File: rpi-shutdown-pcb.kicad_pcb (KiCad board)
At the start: 2 copper layers, 40.5 x 22 mm, 16 parts, among them IC1 ATTINY85-P, P1 CONN_01X03, P2 CONN_01X02, Q1 MOSFET_N_(2N7002P,215), Q2 MOSFET_N_(2N7002P,215), Q3 SI2369DS-T1-GE3, U1 LM3480-3.3

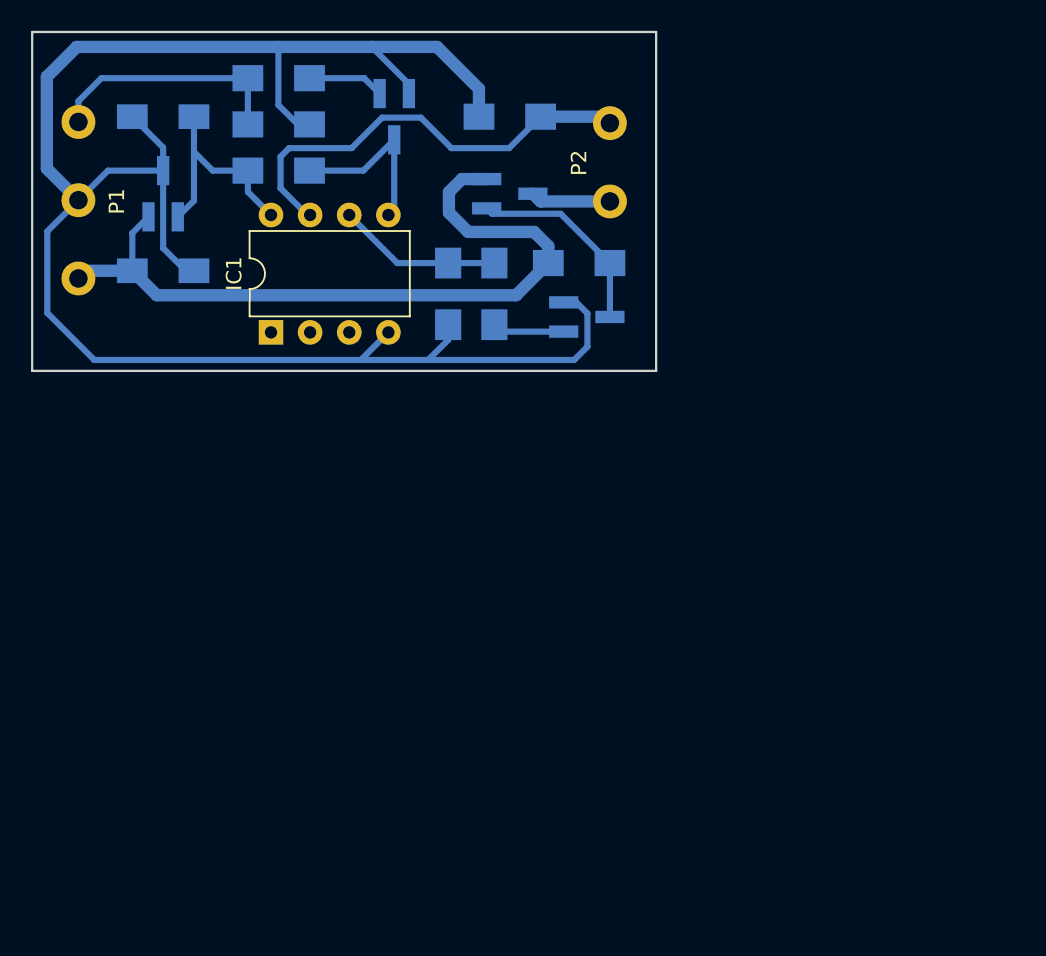
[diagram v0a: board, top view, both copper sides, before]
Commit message: Finished PCB layout.  Ready to try routing.
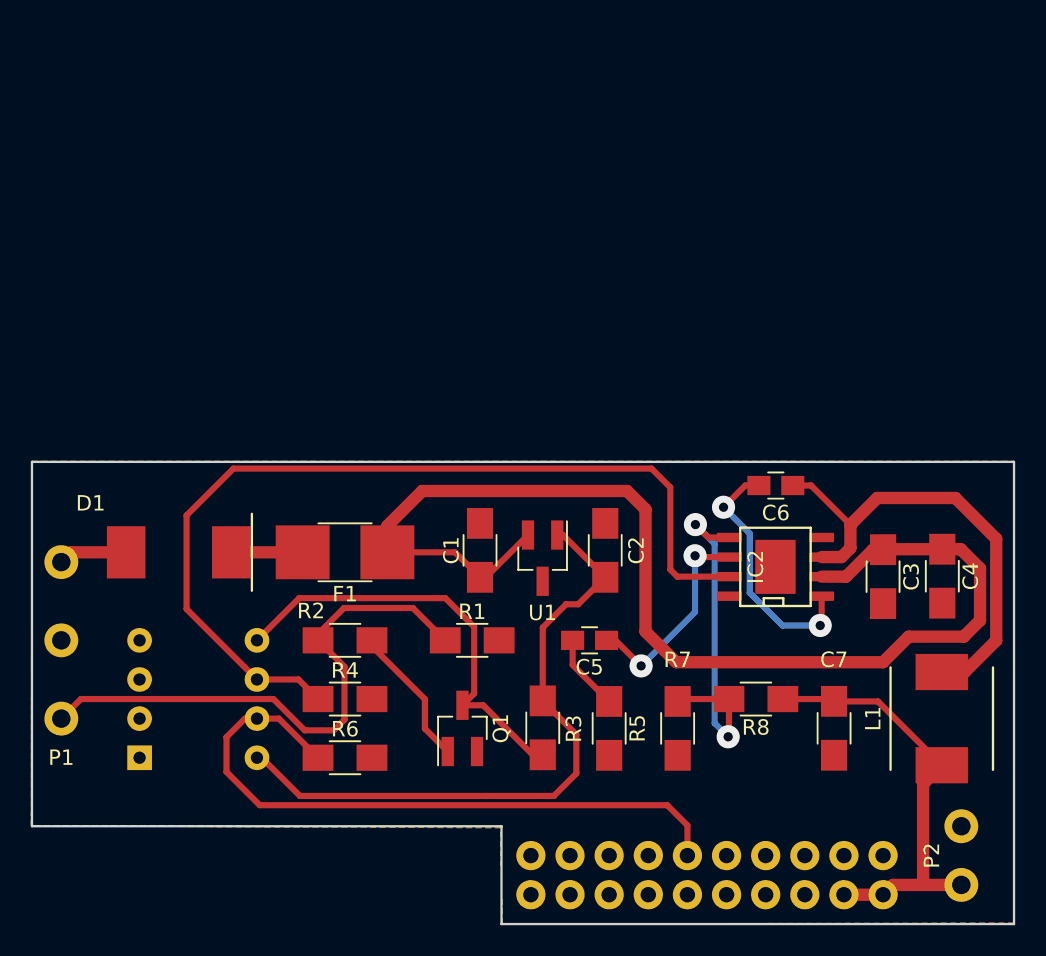
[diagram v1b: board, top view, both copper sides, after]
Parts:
- removed Q2: MOSFET_N_(2N7002P,215), TO_SOT_Packages_SMD:SOT-23_Handsoldering
- removed Q3: SI2369DS-T1-GE3, TO_SOT_Packages_SMD:SOT-23_Handsoldering
- added C3: 10uF, rpi-shutdown-pcb:R_1206_HandSoldering_(narrow), F.Cu at (189.2, 106.4)
- added C4: 10uF, rpi-shutdown-pcb:R_1206_HandSoldering_(narrow), F.Cu at (193.1, 106.3)
- added C5: 3.9nF, rpi-shutdown-pcb:C_0805_HandSoldering_(narrow), F.Cu at (170.2, 110.5)
- added C6: 10nF, rpi-shutdown-pcb:C_0805_HandSoldering_(narrow), F.Cu at (182.3, 100.4)
- added C7: 33uF, rpi-shutdown-pcb:R_1206_HandSoldering_(narrow), F.Cu at (186.1, 116.2)
- added CONN_1: CONN_02X10, rpi-shutdown-pcb:HEADER_20_PIN_FEMALE_(PPTC102LFBN-RC), B.Cu at (189.2, 124.5)
- added D1: D_Schottky, rpi-shutdown-pcb:DO-214AB, F.Cu at (143.5, 104.8)
- added F1: Polyfuse, rpi-shutdown-pcb:R_1812_HandSoldering, F.Cu at (154.3, 104.8)
- added IC2: STEP_DOWN_CONVERTER_(MP2307), rpi-shutdown-pcb:SOIC8N_(EXPOSED_PAD), F.Cu at (182.2, 105.7)
- added L1: 10uH, rpi-shutdown-pcb:INDUCTOR_10uH_(ASPI-0630LR), F.Cu at (193.0, 115.6)
- added R8: 10k, rpi-shutdown-pcb:R_1206_HandSoldering_(narrow), F.Cu at (181.0, 114.3)
- C1, C2: footprint Capacitors_SMD:C_1206_HandSoldering -> rpi-shutdown-pcb:R_1206_HandSoldering_(narrow); moved to F.Cu
- IC1: moved to B.Cu
- Q1, U1: moved to F.Cu
- R1, R2, R3, R4, R6: footprint Resistors_SMD:R_1206_HandSoldering -> rpi-shutdown-pcb:R_1206_HandSoldering_(narrow); moved to F.Cu
- R5: value 150 -> 6.8K; footprint Resistors_SMD:R_1206_HandSoldering -> rpi-shutdown-pcb:R_1206_HandSoldering_(narrow); moved to F.Cu
- R7: value 0.1 -> 2.2K; footprint Resistors_SMD:R_1206_HandSoldering -> rpi-shutdown-pcb:R_1206_HandSoldering_(narrow); moved to F.Cu
- moved P2 49.9 mm to (194.3, 126.4)
- moved R7 41.2 mm to (175.9, 116.2), turned to 270 degrees
- moved C2 40.2 mm to (171.2, 104.6), turned to 90 degrees
- moved R3 40.0 mm to (167.1, 116.2), turned to 270 degrees
- moved Q1 40.0 mm to (161.9, 116.2), turned to 90 degrees
- moved R2 36.7 mm to (154.3, 110.5)
- moved R1 35.8 mm to (162.6, 110.5)
- moved R6 35.5 mm to (154.3, 118.1)
- moved U1 34.2 mm to (167.1, 105.2), turned to 270 degrees
- moved R5 29.2 mm to (171.4, 116.2), turned to 270 degrees
- moved IC1 28.9 mm to (141.0, 118.1), turned to 0 degrees
- moved C1 27.4 mm to (163.1, 104.6), turned to 90 degrees
- moved R4 27.1 mm to (154.3, 114.3), turned to 0 degrees
- moved P1 18.4 mm to (135.9, 105.4), turned to 270 degrees
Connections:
- IC1 pad 7: Net-(IC1-Pad7) -> Net-(CONN_1-Pad11)
- P1 pad 1: Net-(C1-Pad1) -> Net-(D1-Pad2)
- P2 pad 2: Net-(IC1-Pad7) -> GND
- R5 pad 2: Net-(IC1-Pad6) -> GND
- R6 pad 1: Net-(C1-Pad1) -> Net-(CONN_1-Pad11)
- R6 pad 2: Net-(Q2-Pad3) -> GND
- R7 pad 1: GND -> Net-(IC2-Pad5)
- R7 pad 2: Net-(IC1-Pad7) -> GND
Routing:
- net GND: track 124.0 -> 1.33 mm
- net Net-(IC1-Pad6): track 10.7 -> 59.6 mm
- net Net-(CONN_1-Pad11): track 0.00 -> 43.1 mm
- net Net-(C6-Pad1): track 0.00 -> 32.1 mm
- net Net-(IC1-Pad7): track 29.5 -> 0.00 mm
- net Net-(C1-Pad1): track 48.8 -> 77.3 mm
- net Net-(C2-Pad1): track 14.4 -> 42.5 mm
- net Net-(IC2-Pad5): track 0.00 -> 23.1 mm, vias 0 -> 2
- net Net-(C7-Pad1): track 5.21 -> 28.2 mm
- net Net-(P1-Pad3): track 16.0 -> 36.1 mm
- net Net-(IC1-Pad5): track 11.4 -> 28.0 mm
- net Net-(C6-Pad2): track 0.00 -> 16.5 mm, vias 0 -> 2
- net Net-(C5-Pad1): track 0.00 -> 13.8 mm, vias 0 -> 2
- net Net-(Q2-Pad3): track 13.0 -> 0.00 mm
- net Net-(D1-Pad1): track 0.00 -> 4.64 mm
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- added copper zone on B.Cu, net GND
- added copper zone on F.Cu, net GND
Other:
- board size 40.5 x 22 mm -> 63.7 x 30 mm
